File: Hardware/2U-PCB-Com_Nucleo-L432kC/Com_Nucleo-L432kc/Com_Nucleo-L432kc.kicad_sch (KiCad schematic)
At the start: 40 parts, among them IC1 PCI_EXPRESS_CARD, J1 Bus Standard, J2 I2C_Grove, J3 I2C_Grove, J4 Conn_01x08, J5 Conn_01x08, J6 Conn_01x15, J7 Conn_01x15, J8 I2C_Grove, J9 I2C_Grove, U1 7404

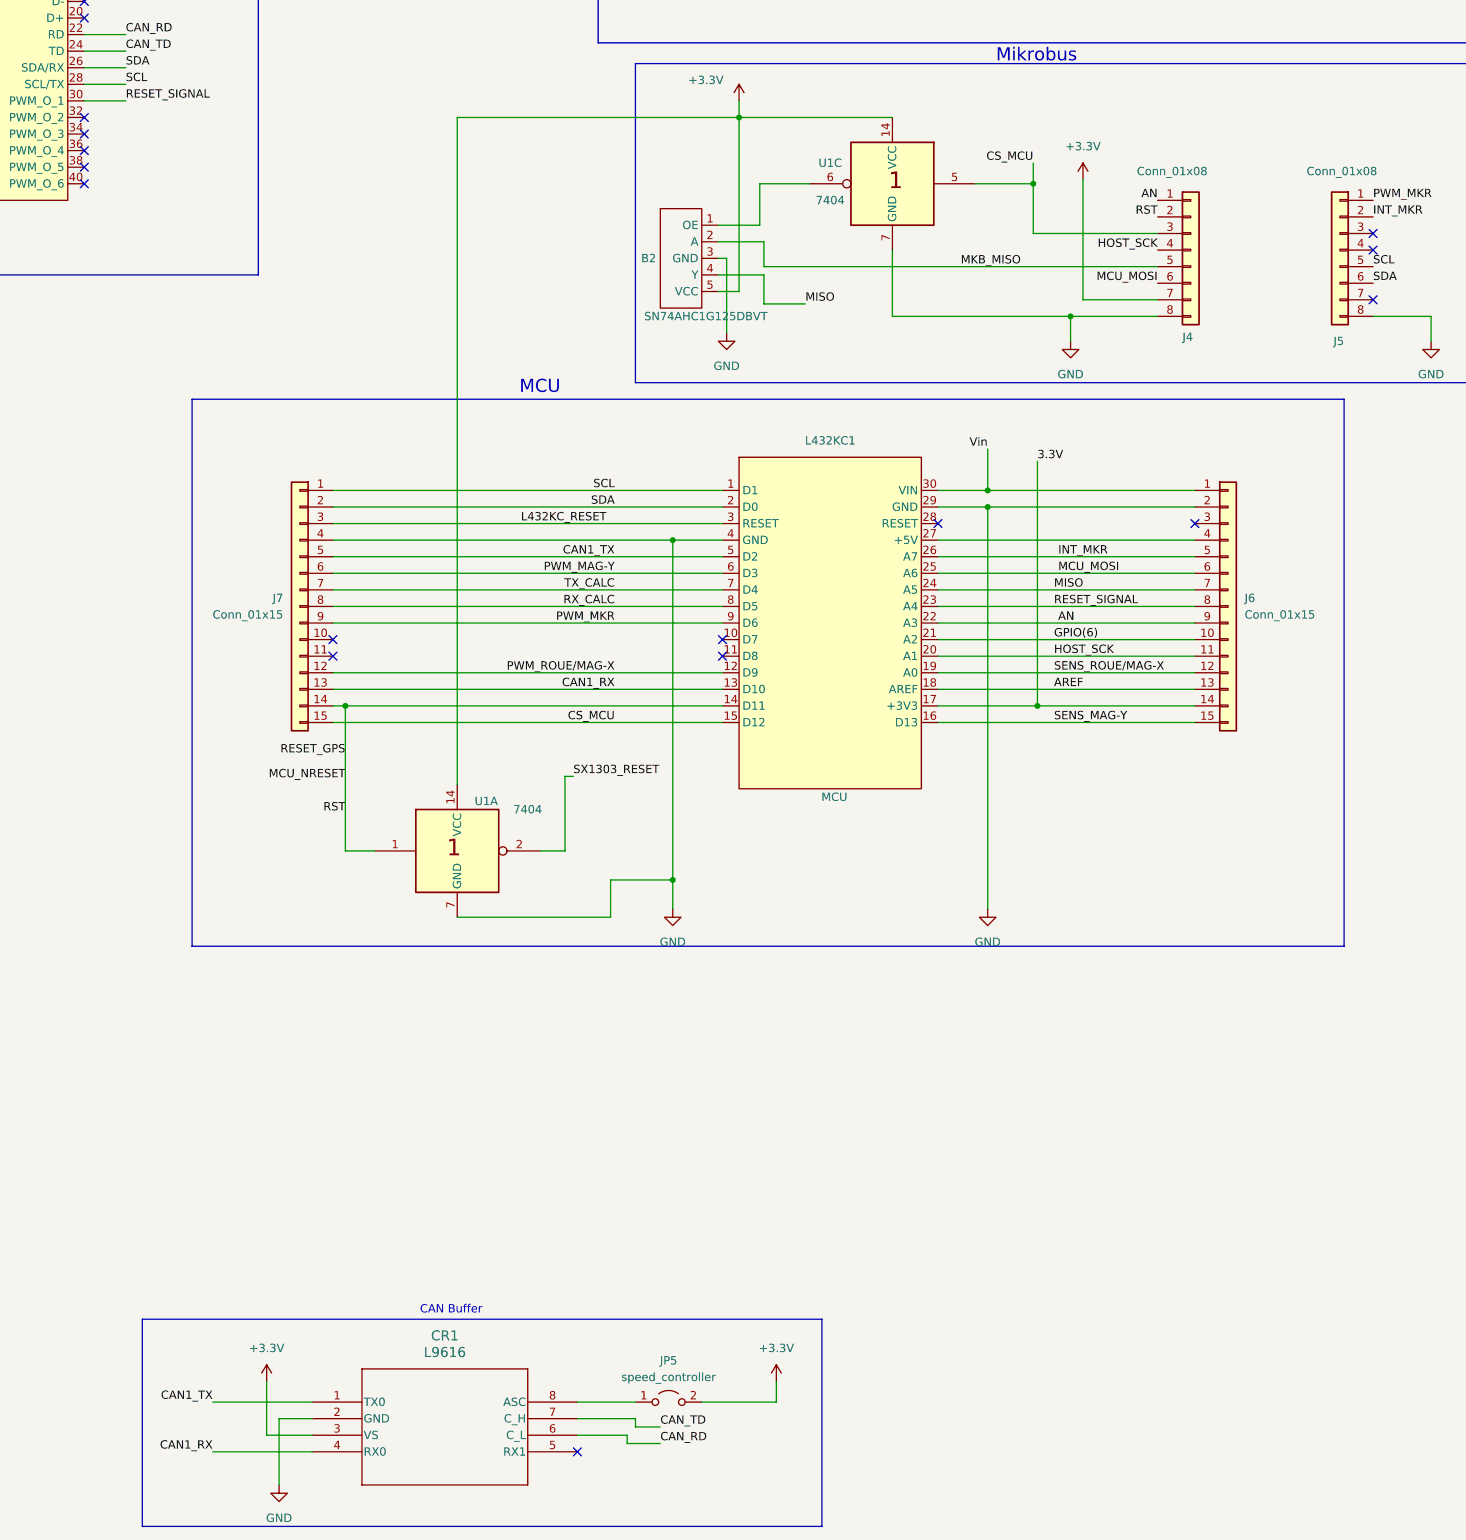
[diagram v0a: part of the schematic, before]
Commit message: First version for fabrication
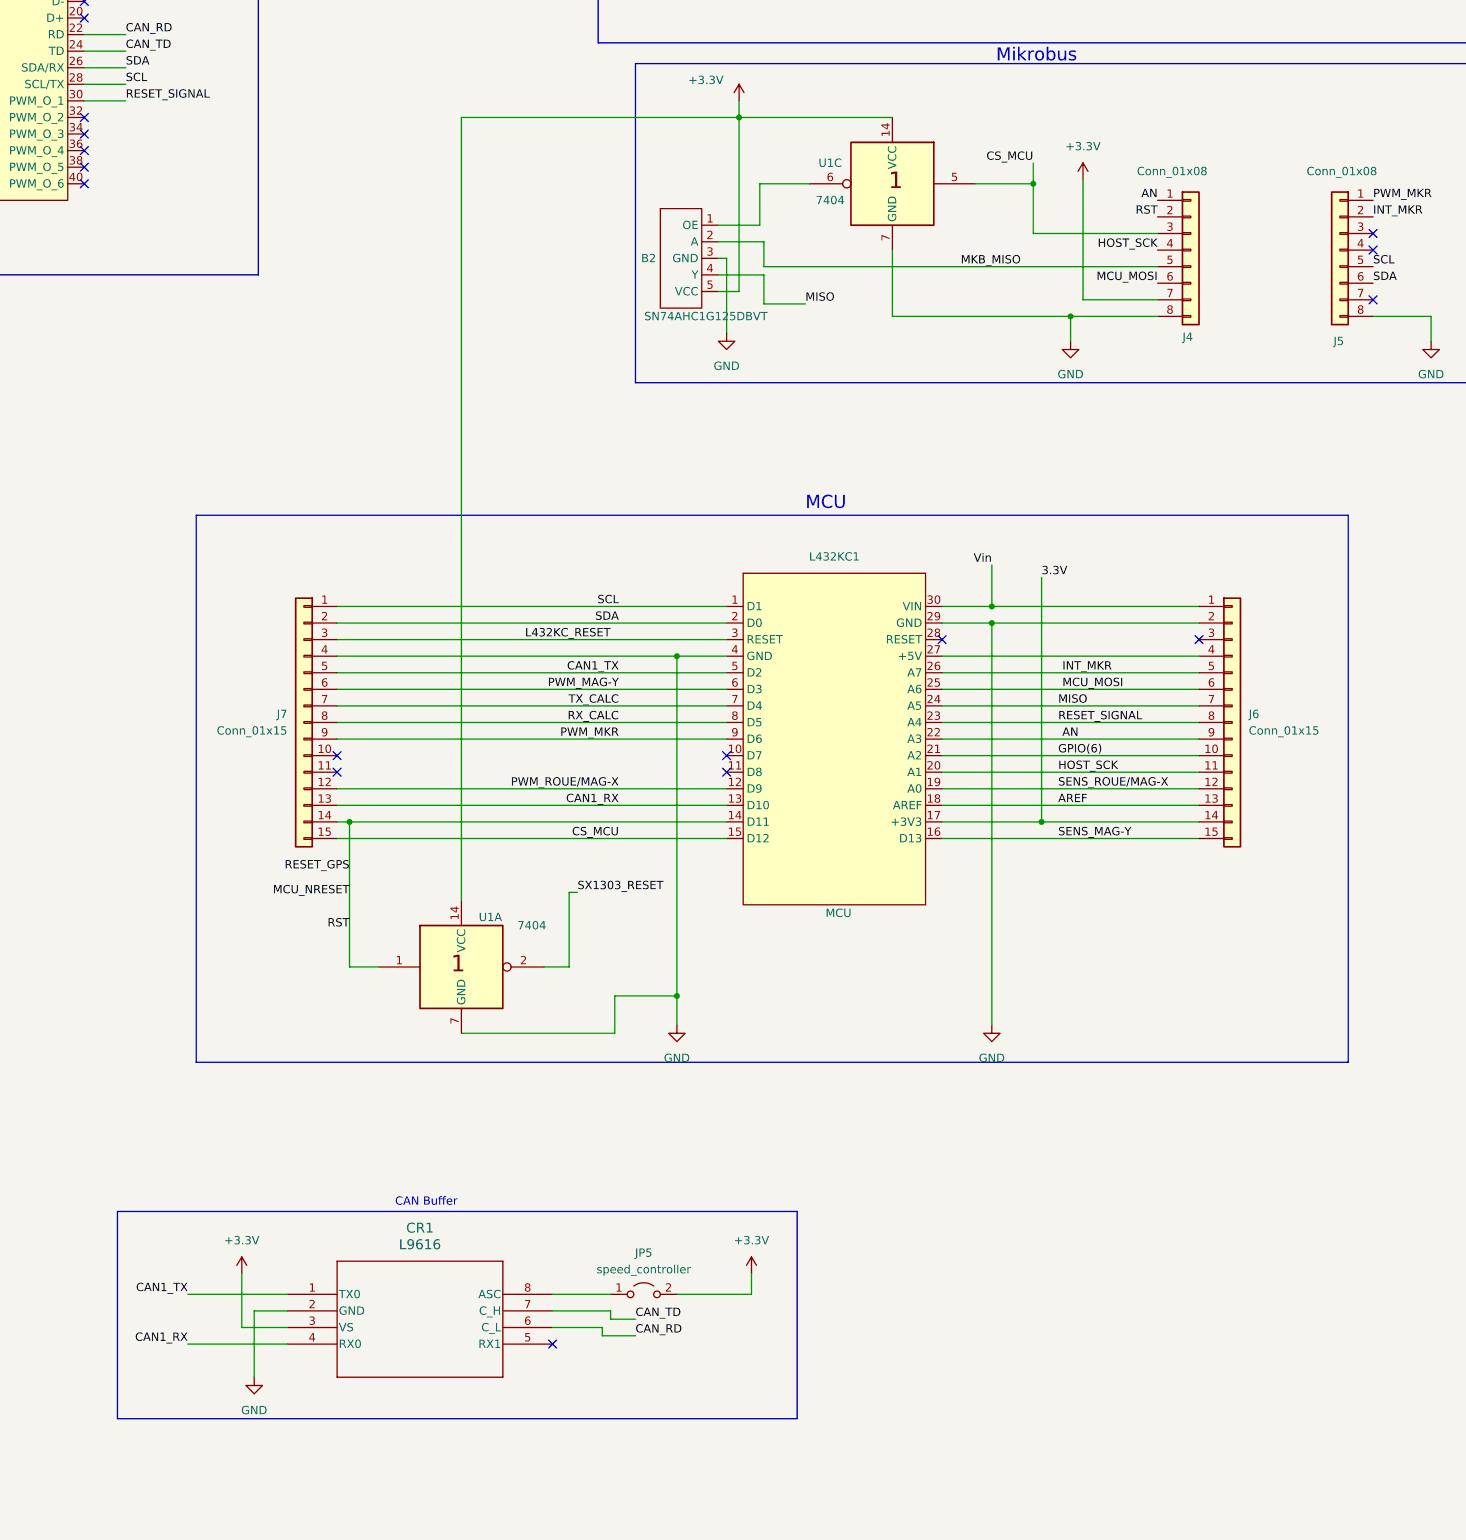
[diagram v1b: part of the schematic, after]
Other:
- moved on the sheet: CR1, J6, J7, JP5, L432KC1, U1A
